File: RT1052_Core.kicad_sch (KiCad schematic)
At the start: 8 parts, among them IC1 SN74AHCT1G125DCK3, U1 M1052-16F128AWI-T

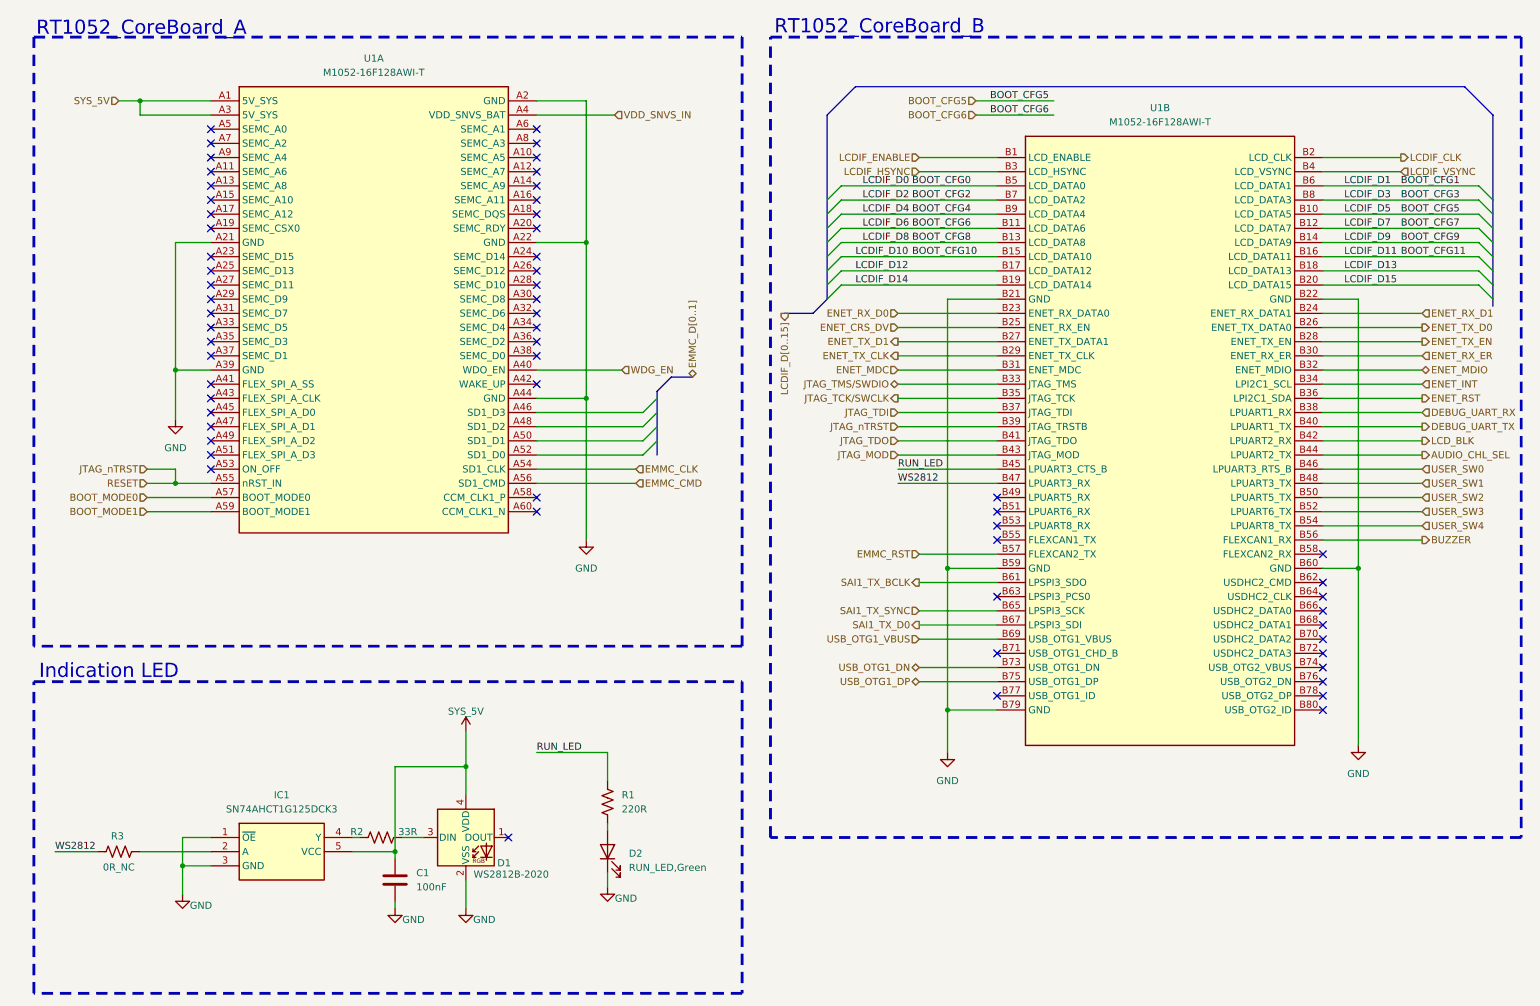
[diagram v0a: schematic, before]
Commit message: 2026 08 24 画图完成，准备生产
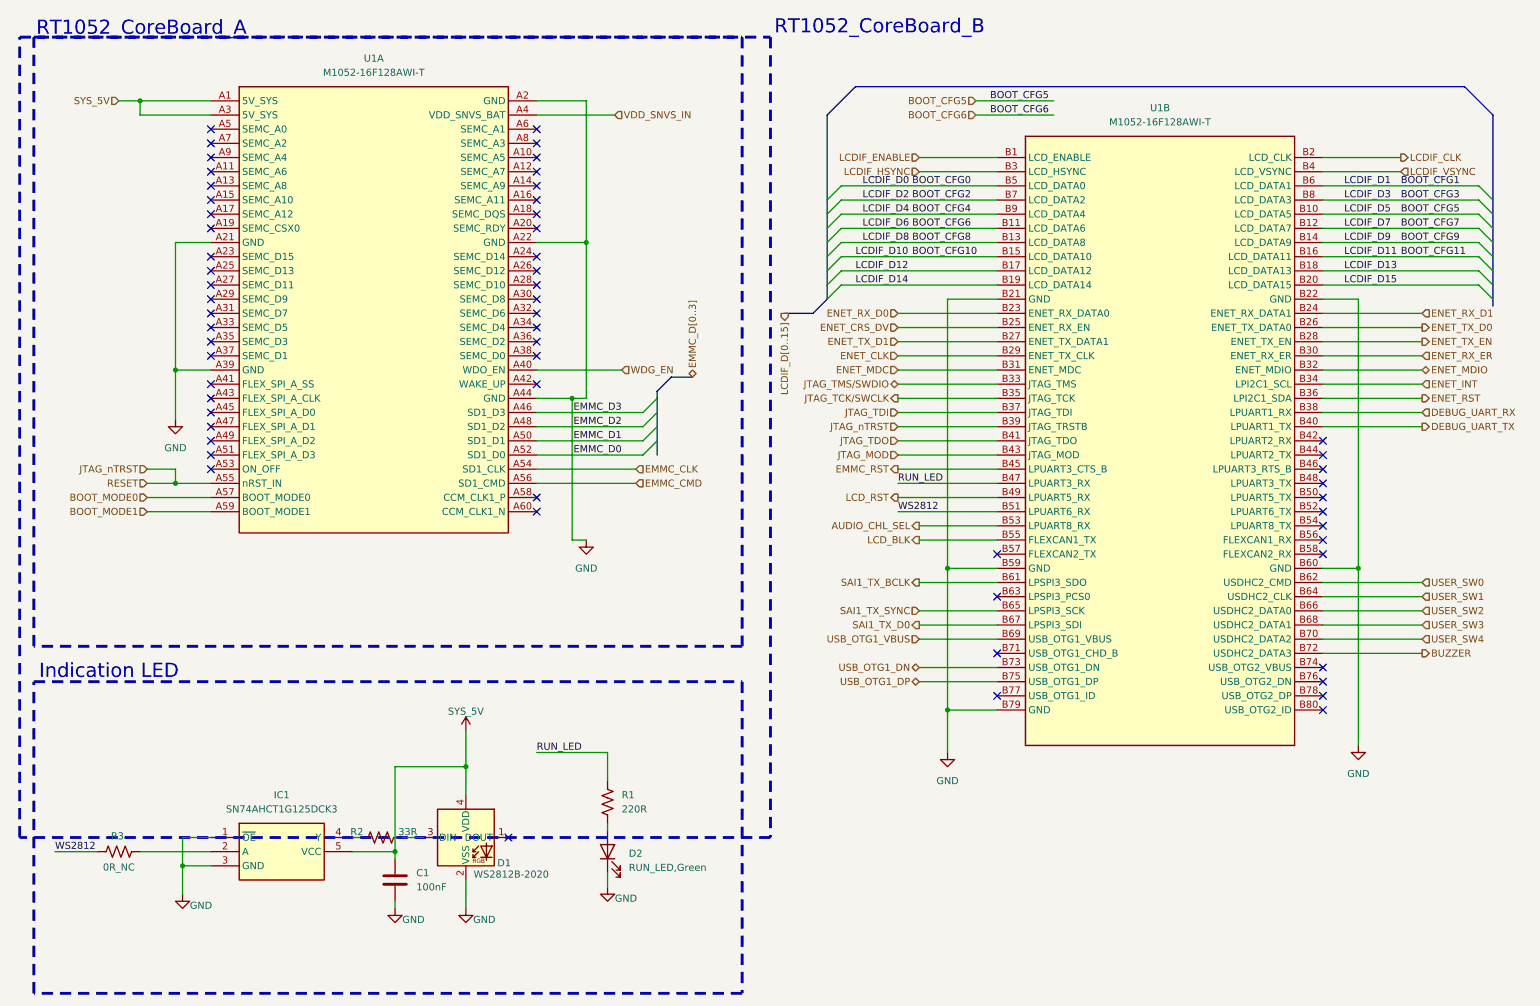
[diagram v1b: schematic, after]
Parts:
- U1: footprint (none) -> UPT:M1052-16F128AWI-T
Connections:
- net AUDIO_CHL_SEL: now also U1.B53 (LPUART8_RX); no longer U1.B44 (LPUART2_TX)
- net BUZZER: now also U1.B72 (USDHC2_DATA3); no longer U1.B56 (FLEXCAN1_RX)
- net EMMC_RST: now also U1.B45 (LPUART3_CTS_B); no longer U1.B57 (FLEXCAN2_TX)
- net LCD_BLK: now also U1.B55 (FLEXCAN1_TX); no longer U1.B42 (LPUART2_RX)
- net RUN_LED: now also U1.B47 (LPUART3_RX); no longer U1.B45 (LPUART3_CTS_B)
- net USER_SW0: now also U1.B62 (USDHC2_CMD); no longer U1.B46 (LPUART3_RTS_B)
- net USER_SW1: now also U1.B64 (USDHC2_CLK); no longer U1.B48 (LPUART3_TX)
- net USER_SW2: now also U1.B66 (USDHC2_DATA0); no longer U1.B50 (LPUART5_TX)
- net USER_SW3: now also U1.B68 (USDHC2_DATA1); no longer U1.B52 (LPUART6_TX)
- net USER_SW4: now also U1.B70 (USDHC2_DATA2); no longer U1.B54 (LPUART8_TX)
- net WS2812: now also U1.B51 (LPUART6_RX); no longer U1.B47 (LPUART3_RX)
- net EMMC_D3: now reaches U1.A46 (SD1_D3)
- net EMMC_D2: now reaches U1.A48 (SD1_D2)
- net EMMC_D1: now reaches U1.A50 (SD1_D1)
- net EMMC_D0: now reaches U1.A52 (SD1_D0)
- net LCD_RST: now reaches U1.B49 (LPUART5_RX)
- net ENET_TX_CLK renamed ENET_CLK
- no-connect marks 61 -> 60
